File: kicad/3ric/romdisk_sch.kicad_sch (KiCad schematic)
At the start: 48 parts

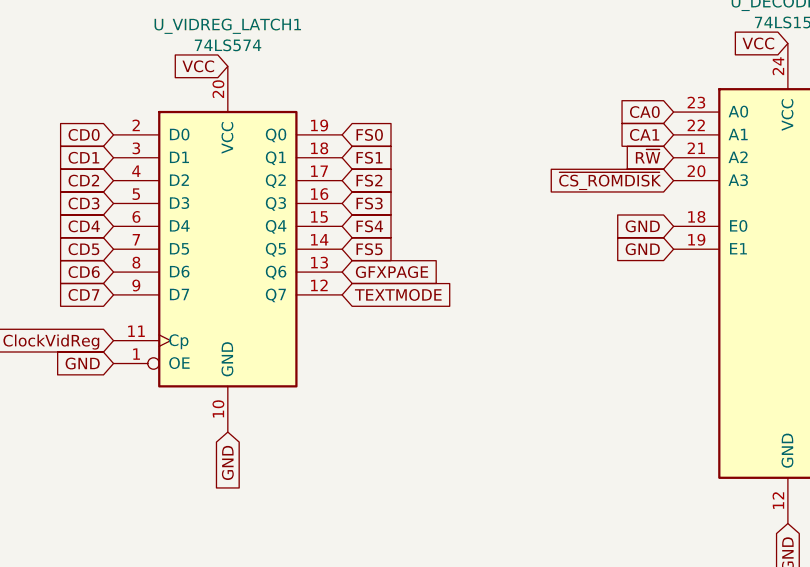
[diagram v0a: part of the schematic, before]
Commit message: updates to logisim project and schematics
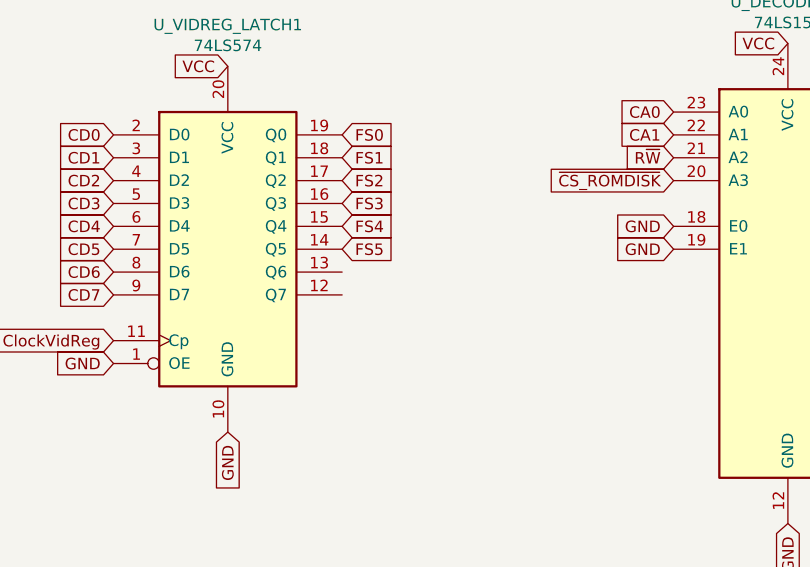
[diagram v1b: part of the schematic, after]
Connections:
- net GFXPAGE: no longer U_VIDREG_LATCH1.13 (Q6)
- net TEXTMODE: no longer U_VIDREG_LATCH1.12 (Q7)
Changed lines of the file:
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@@
-    )
-  )
-  (global_label "TEXTMODE" (shape input) (at 107.95 130.81 0) (fields_autoplaced)
-    (effects (font (size 1.27 1.27)) (justify left))
-    (property "Intersheet References" "${INTERSHEET_REFS}" (id 0) (at 119.8579 130.7306 0)
-      (effects (font (size 1.27 1.27)) (justify left) hide)
     )
   )
@@
     )
   )
-  (global_label "GFXPAGE" (shape input) (at 107.95 128.27 0) (fields_autoplaced)
-    (effects (font (size 1.27 1.27)) (justify left))
-    (property "Intersheet References" "${INTERSHEET_REFS}" (id 0) (at 118.7088 128.1906 0)
-      (effects (font (size 1.27 1.27)) (justify left) hide)
-    )
-  )

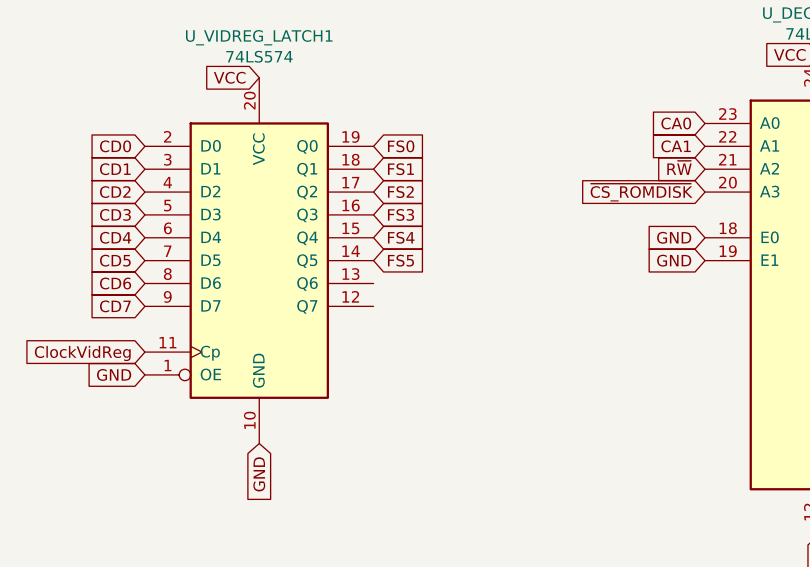
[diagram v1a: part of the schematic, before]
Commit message: update schematics
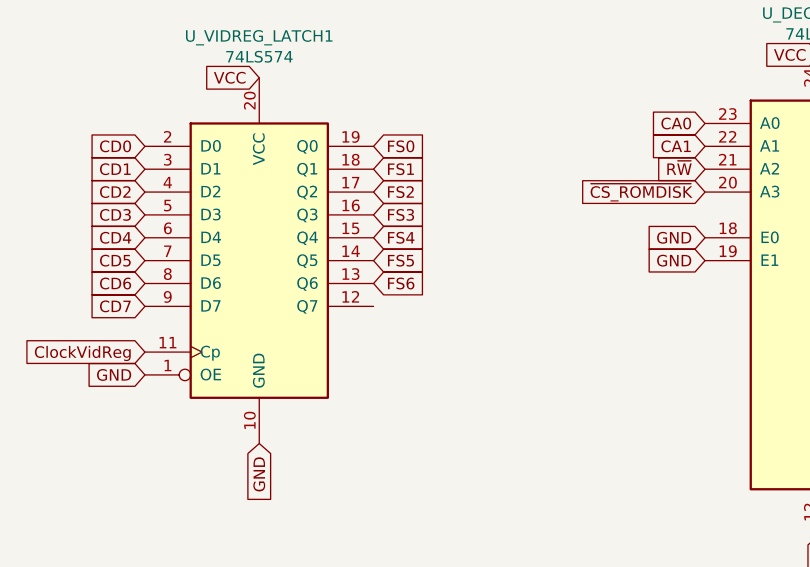
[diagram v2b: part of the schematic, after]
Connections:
- net FS6: now reaches U_VIDREG_LATCH1.13 (Q6)
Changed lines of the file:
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@@
 (kicad_sch (version 20211123) (generator eeschema)
   (paper "A4")
-  (no_connect (at 170.18 130.81))
   (no_connect (at 170.18 148.59))
   (no_connect (at 170.18 140.97))
   (no_connect (at 170.18 133.35))
   (no_connect (at 170.18 135.89))
+  (no_connect (at 170.18 130.81))
   (no_connect (at 170.18 146.05))
   (no_connect (at 170.18 143.51))
@@
     )
   )
+  (global_label "~{RomDiskOE}" (shape input) (at 170.18 128.27 0) (fields_autoplaced)
+    (effects (font (size 1.27 1.27)) (justify left))
+    (property "Intersheet References" "${INTERSHEET_REFS}" (id 0) (at -8.89 11.43 0)
+      (effects (font (size 1.27 1.27)) hide)
+    )
+  )
   (global_label "GND" (shape input) (at 209.55 60.96 180) (fields_autoplaced)
     (effects (font (size 1.27 1.27)) (justify right))
@@
     )
   )
+  (global_label "FS6" (shape input) (at 107.95 128.27 0) (fields_autoplaced)
+    (effects (font (size 1.27 1.27)) (justify left))
+    (property "Intersheet References" "${INTERSHEET_REFS}" (id 0) (at 113.8707 128.1906 0)
+      (effects (font (size 1.27 1.27)) (justify left) hide)
+    )
+  )
   (global_label "RA8" (shape input) (at 30.48 109.22 180) (fields_autoplaced)
     (effects (font (size 1.27 1.27)) (justify right))
@@
     )
   )
-  (global_label "~{RomDiskOE}" (shape input) (at 170.18 128.27 0) (fields_autoplaced)
-    (effects (font (size 1.27 1.27)) (justify left))
-    (property "Intersheet References" "${INTERSHEET_REFS}" (id 0) (at -8.89 11.43 0)
-      (effects (font (size 1.27 1.27)) hide)
-    )
-  )
